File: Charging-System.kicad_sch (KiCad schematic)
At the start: 6 parts

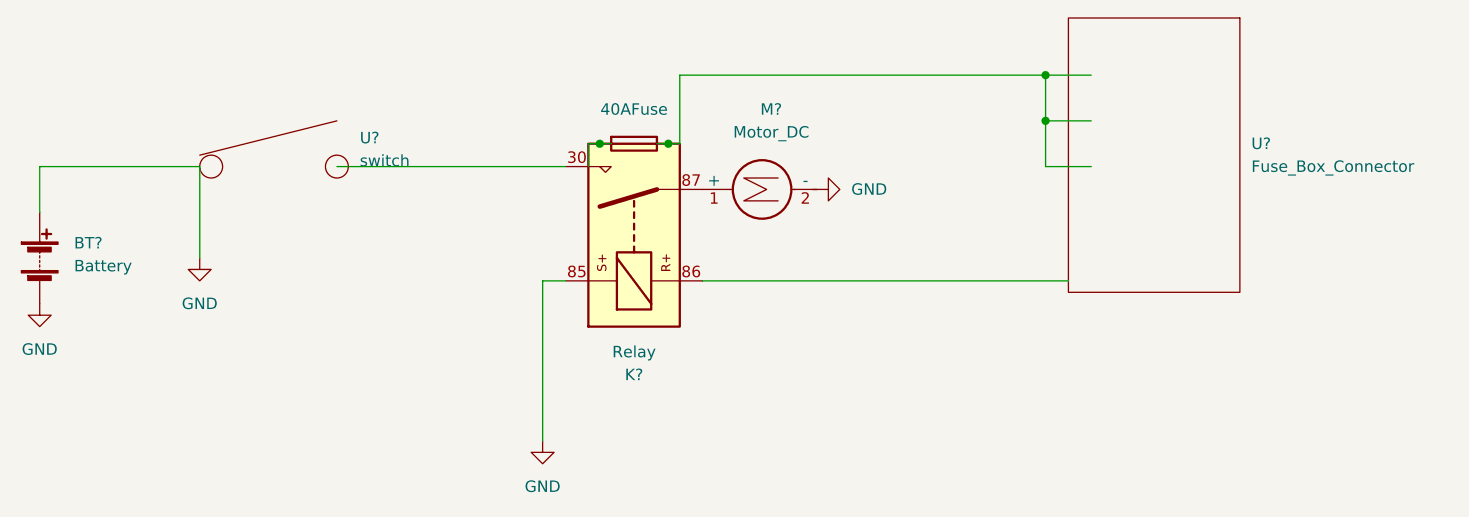
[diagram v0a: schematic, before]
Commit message: Changes to DTM Dash
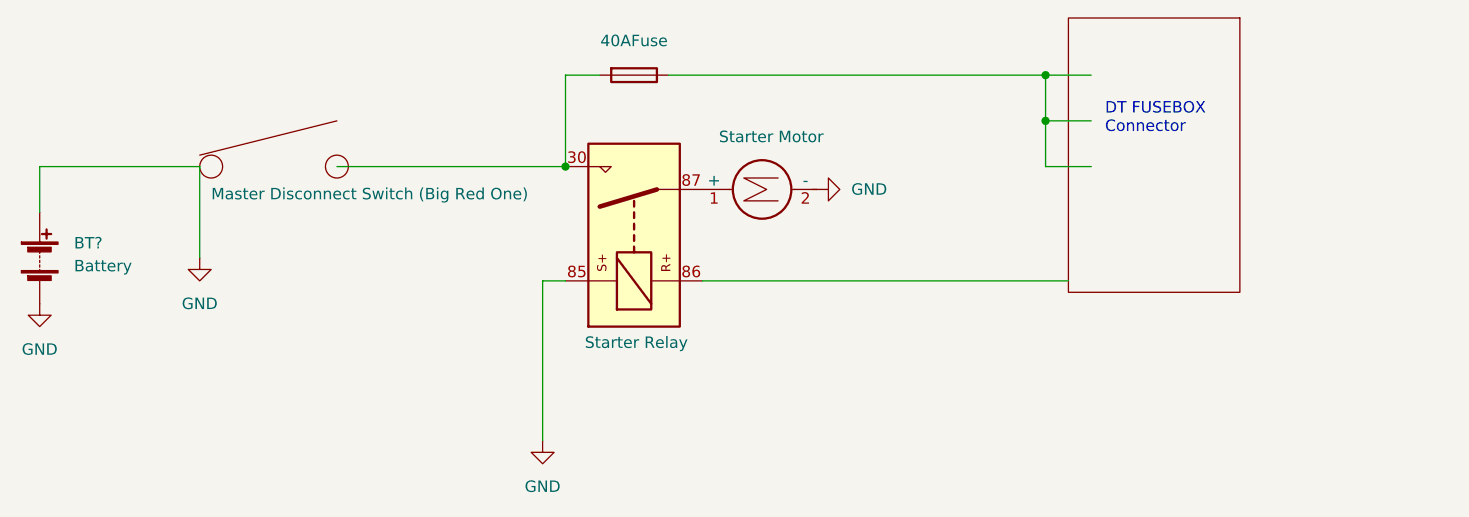
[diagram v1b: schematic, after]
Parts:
- K?: value Relay -> Starter Relay
- M?: value Motor_DC -> Starter Motor
- U?: value switch -> Master Disconnect Switch (Big Red One)
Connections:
- net at K?.30: now also F?.2
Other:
- note added: "DT FUSEBOX Connector"
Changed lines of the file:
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@@
   (junction (at 192.532 62.992) (diameter 0) (color 0 0 0 0)
   )
+  (junction (at 139.192 73.152) (diameter 0) (color 0 0 0 0)
+  )
   (junction (at 192.532 68.072) (diameter 0) (color 0 0 0 0)
-  )
-  (junction (at 150.622 70.612) (diameter 0) (color 0 0 0 0)
-  )
-  (junction (at 143.002 70.612) (diameter 0) (color 0 0 0 0)
   )
   (wire (pts (xy 197.612 73.152) (xy 192.532 73.152))
@@
     (stroke (width 0) (type default) (color 0 0 0 0))
   )
-  (wire (pts (xy 141.732 70.612) (xy 141.732 73.152))
-    (stroke (width 0) (type default) (color 0 0 0 0))
-  )
-  (wire (pts (xy 143.002 70.612) (xy 141.732 70.612))
-    (stroke (width 0) (type default) (color 0 0 0 0))
-  )
   (wire (pts (xy 136.652 85.852) (xy 136.652 103.632))
-    (stroke (width 0) (type default) (color 0 0 0 0))
-  )
-  (wire (pts (xy 150.622 70.612) (xy 151.892 70.612))
-    (stroke (width 0) (type default) (color 0 0 0 0))
-  )
-  (wire (pts (xy 149.352 70.612) (xy 150.622 70.612))
     (stroke (width 0) (type default) (color 0 0 0 0))
   )
@@
     (stroke (width 0) (type default) (color 0 0 0 0))
   )
-  (wire (pts (xy 113.792 73.152) (xy 139.192 73.152))
+  (wire (pts (xy 139.192 62.992) (xy 143.002 62.992))
     (stroke (width 0) (type default) (color 0 0 0 0))
   )
-  (wire (pts (xy 151.892 62.992) (xy 151.892 70.612))
+  (wire (pts (xy 113.792 73.152) (xy 139.192 73.152))
     (stroke (width 0) (type default) (color 0 0 0 0))
   )
@@
     (stroke (width 0) (type default) (color 0 0 0 0))
   )
-  (wire (pts (xy 144.272 70.612) (xy 143.002 70.612))
-    (stroke (width 0) (type default) (color 0 0 0 0))
-  )
-  (wire (pts (xy 151.892 62.992) (xy 192.532 62.992))
+  (wire (pts (xy 139.192 62.992) (xy 139.192 73.152))
     (stroke (width 0) (type default) (color 0 0 0 0))
   )
@@
     (stroke (width 0) (type default) (color 0 0 0 0))
   )
+  (wire (pts (xy 150.622 62.992) (xy 192.532 62.992))
+    (stroke (width 0) (type default) (color 0 0 0 0))
+  )
   (wire (pts (xy 139.192 85.852) (xy 136.652 85.852))
     (stroke (width 0) (type default) (color 0 0 0 0))
+  )
+  (text "DT FUSEBOX\nConnector\n" (at 199.136 69.596 0)
+    (effects (font (size 1.27 1.27)) (justify left bottom))
   )
   (symbol (lib_id "symbols:Fuse_Box_Connector") (at 205.232 70.612 270) (unit 1)
     (in_bom yes) (on_board yes) (fields_autoplaced)
     (property "Reference" "U?" (id 0) (at 215.392 70.6119 90)
-      (effects (font (size 1.27 1.27)) (justify left))
+      (effects (font (size 1.27 1.27)) (justify left) hide)
     )
-    (property "Value" "Fuse_Box_Connector" (id 1) (at 215.392 73.1519 90)
-      (effects (font (size 1.27 1.27)) (justify left))
+    (property "Value" "Fuse_Box_Connector" (id 1) (at 215.9 71.8819 90)
+      (effects (font (size 1.27 1.27)) (justify left) hide)
     )
     (property "Footprint" "" (id 2) (at 205.232 70.612 0)
@@
   )
   (symbol (lib_id "symbols:switch") (at 106.172 73.152 0) (unit 1)
-    (in_bom yes) (on_board yes) (fields_autoplaced)
-    (property "Reference" "U?" (id 0) (at 116.332 69.9769 0)
-      (effects (font (size 1.27 1.27)) (justify left))
+    (in_bom yes) (on_board yes)
+    (property "Reference" "U?" (id 0) (at 116.84 69.9769 0)
+      (effects (font (size 1.27 1.27)) (justify left) hide)
     )
-    (property "Value" "switch" (id 1) (at 116.332 72.5169 0)
+    (property "Value" "Master Disconnect Switch (Big Red One)" (id 1) (at 99.822 76.2 0)
       (effects (font (size 1.27 1.27)) (justify left))
     )
@@
   (symbol (lib_id "Motor:Motor_DC") (at 159.512 75.692 90) (unit 1)
     (in_bom yes) (on_board yes) (fields_autoplaced)
-    (property "Reference" "M?" (id 0) (at 162.052 66.802 90))
-    (property "Value" "Motor_DC" (id 1) (at 162.052 69.342 90))
+    (property "Reference" "M?" (id 0) (at 162.052 67.31 90)
+      (effects (font (size 1.27 1.27)) hide)
+    )
+    (property "Value" "Starter Motor" (id 1) (at 162.052 69.85 90))
     (property "Footprint" "" (id 2) (at 161.798 75.692 0)
       (effects (font (size 1.27 1.27)) hide)
@@
   )
   (symbol (lib_id "SCR23 Library:Relay") (at 146.7485 80.9117 180) (unit 1)
-    (in_bom yes) (on_board yes) (fields_autoplaced)
-    (property "Reference" "K?" (id 0) (at 146.812 96.2914 0))
-    (property "Value" "Relay" (id 1) (at 146.812 93.7514 0))
+    (in_bom yes) (on_board yes)
+    (property "Reference" "K?" (id 0) (at 146.812 64.77 0)
+      (effects (font (size 1.27 1.27)) hide)
+    )
+    (property "Value" "Starter Relay" (id 1) (at 147.066 92.71 0))
     (property "Footprint" "" (id 2) (at 113.0935 79.6417 0)
       (effects (font (size 1.27 1.27)) hide)
@@
     (pin "1")
   )
-  (symbol (lib_id "Device:Fuse") (at 146.812 70.612 270) (unit 1)
+  (symbol (lib_id "Device:Fuse") (at 146.812 62.992 270) (unit 1)
     (in_bom yes) (on_board yes) (fields_autoplaced)
-    (property "Reference" "F?" (id 0) (at 146.812 64.262 90)
+    (property "Reference" "F?" (id 0) (at 146.812 56.642 90)
       (effects (font (size 1.27 1.27)) hide)
     )
-    (property "Value" "40AFuse" (id 1) (at 146.812 66.802 90))
-    (property "Footprint" "" (id 2) (at 146.812 68.834 90)
+    (property "Value" "40AFuse" (id 1) (at 146.812 59.182 90))
+    (property "Footprint" "" (id 2) (at 146.812 61.214 90)
       (effects (font (size 1.27 1.27)) hide)
     )
-    (property "Datasheet" "~" (id 3) (at 146.812 70.612 0)
+    (property "Datasheet" "~" (id 3) (at 146.812 62.992 0)
       (effects (font (size 1.27 1.27)) hide)
     )

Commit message: Create new top level
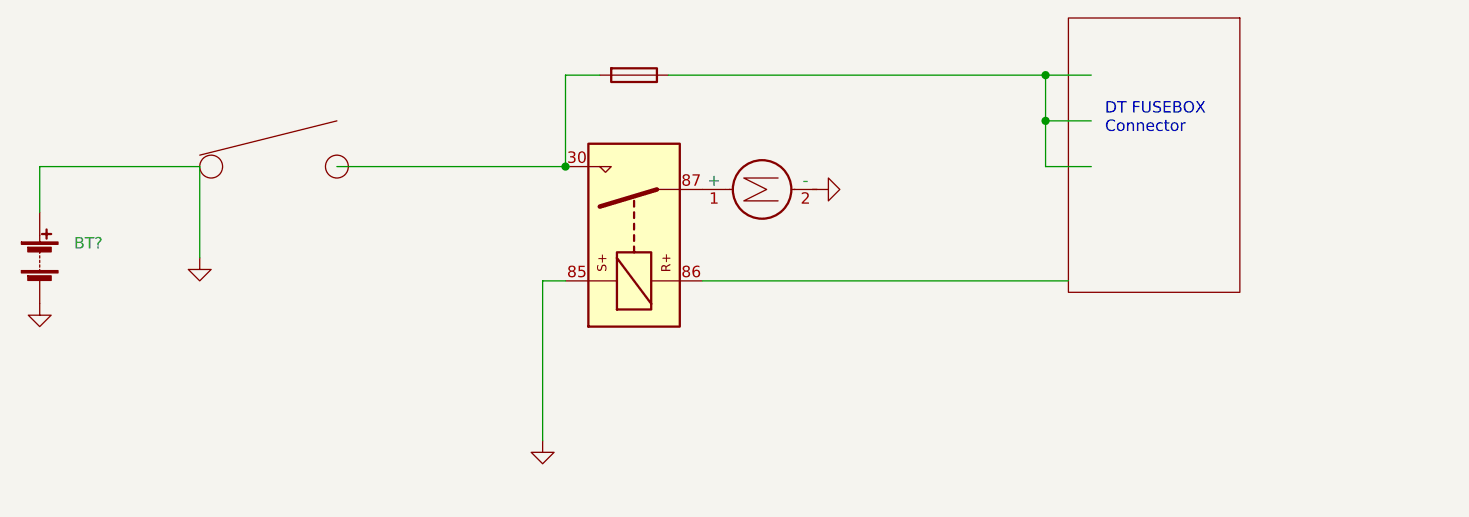
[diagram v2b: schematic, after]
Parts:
- BT?: value Battery -> (none)
- F?: value 40AFuse -> (none)
- K?: value Starter Relay -> (none)
- M?: value Starter Motor -> (none)
- U?: value Fuse_Box_Connector -> (none)
- U?: value Master Disconnect Switch (Big Red One) -> (none)
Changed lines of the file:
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@@
       (effects (font (size 1.27 1.27)) (justify left) hide)
     )
-    (property "Value" "Fuse_Box_Connector" (id 1) (at 215.9 71.8819 90)
+    (property "Value" "" (id 1) (at 215.9 71.8819 90)
       (effects (font (size 1.27 1.27)) (justify left) hide)
     )
@@
       (effects (font (size 1.27 1.27)) (justify left) hide)
     )
-    (property "Value" "Master Disconnect Switch (Big Red One)" (id 1) (at 99.822 76.2 0)
+    (property "Value" "" (id 1) (at 99.822 76.2 0)
       (effects (font (size 1.27 1.27)) (justify left))
     )
@@
       (effects (font (size 1.27 1.27)) hide)
     )
-    (property "Value" "GND" (id 1) (at 170.942 75.6919 90)
+    (property "Value" "" (id 1) (at 170.942 75.6919 90)
       (effects (font (size 1.27 1.27)) (justify right))
     )
@@
       (effects (font (size 1.27 1.27)) hide)
     )
-    (property "Value" "GND" (id 1) (at 80.772 93.472 0))
+    (property "Value" "" (id 1) (at 80.772 93.472 0))
     (property "Footprint" "" (id 2) (at 80.772 88.392 0)
       (effects (font (size 1.27 1.27)) hide)
@@
       (effects (font (size 1.27 1.27)) hide)
     )
-    (property "Value" "GND" (id 1) (at 98.552 88.392 0))
+    (property "Value" "" (id 1) (at 98.552 88.392 0))
     (property "Footprint" "" (id 2) (at 98.552 83.312 0)
       (effects (font (size 1.27 1.27)) hide)
@@
       (effects (font (size 1.27 1.27)) hide)
     )
-    (property "Value" "Starter Motor" (id 1) (at 162.052 69.85 90))
+    (property "Value" "" (id 1) (at 162.052 69.85 90))
     (property "Footprint" "" (id 2) (at 161.798 75.692 0)
       (effects (font (size 1.27 1.27)) hide)
@@
       (effects (font (size 1.27 1.27)) hide)
     )
-    (property "Value" "Starter Relay" (id 1) (at 147.066 92.71 0))
+    (property "Value" "" (id 1) (at 147.066 92.71 0))
     (property "Footprint" "" (id 2) (at 113.0935 79.6417 0)
       (effects (font (size 1.27 1.27)) hide)
@@
       (effects (font (size 1.27 1.27)) hide)
     )
-    (property "Value" "GND" (id 1) (at 136.652 108.712 0))
+    (property "Value" "" (id 1) (at 136.652 108.712 0))
     (property "Footprint" "" (id 2) (at 136.652 103.632 0)
       (effects (font (size 1.27 1.27)) hide)
@@
       (effects (font (size 1.27 1.27)) hide)
     )
-    (property "Value" "40AFuse" (id 1) (at 146.812 59.182 90))
+    (property "Value" "" (id 1) (at 146.812 59.182 90))
     (property "Footprint" "" (id 2) (at 146.812 61.214 90)
       (effects (font (size 1.27 1.27)) hide)
@@
       (effects (font (size 1.27 1.27)) (justify left))
     )
-    (property "Value" "Battery" (id 1) (at 84.582 84.2009 0)
+    (property "Value" "" (id 1) (at 84.582 84.2009 0)
       (effects (font (size 1.27 1.27)) (justify left))
     )

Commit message: HUGE TOP LEVEL
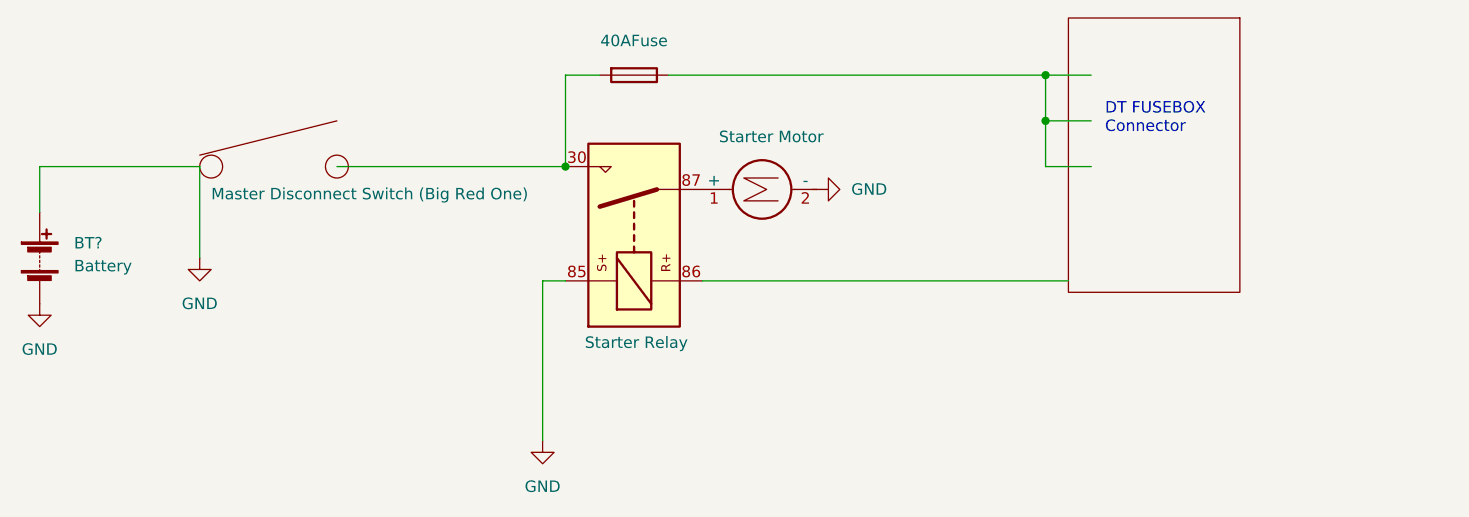
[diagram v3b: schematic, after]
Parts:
- BT?: value (none) -> Battery
- F?: value (none) -> 40AFuse
- K?: value (none) -> Starter Relay
- M?: value (none) -> Starter Motor
- U?: value (none) -> Fuse_Box_Connector
- U?: value (none) -> Master Disconnect Switch (Big Red One)
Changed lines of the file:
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@@
       (effects (font (size 1.27 1.27)) (justify left) hide)
     )
-    (property "Value" "" (id 1) (at 215.9 71.8819 90)
+    (property "Value" "Fuse_Box_Connector" (id 1) (at 215.9 71.8819 90)
       (effects (font (size 1.27 1.27)) (justify left) hide)
     )
@@
       (effects (font (size 1.27 1.27)) (justify left) hide)
     )
-    (property "Value" "" (id 1) (at 99.822 76.2 0)
+    (property "Value" "Master Disconnect Switch (Big Red One)" (id 1) (at 99.822 76.2 0)
       (effects (font (size 1.27 1.27)) (justify left))
     )
@@
       (effects (font (size 1.27 1.27)) hide)
     )
-    (property "Value" "" (id 1) (at 170.942 75.6919 90)
+    (property "Value" "GND" (id 1) (at 170.942 75.6919 90)
       (effects (font (size 1.27 1.27)) (justify right))
     )
@@
       (effects (font (size 1.27 1.27)) hide)
     )
-    (property "Value" "" (id 1) (at 80.772 93.472 0))
+    (property "Value" "GND" (id 1) (at 80.772 93.472 0))
     (property "Footprint" "" (id 2) (at 80.772 88.392 0)
       (effects (font (size 1.27 1.27)) hide)
@@
       (effects (font (size 1.27 1.27)) hide)
     )
-    (property "Value" "" (id 1) (at 98.552 88.392 0))
+    (property "Value" "GND" (id 1) (at 98.552 88.392 0))
     (property "Footprint" "" (id 2) (at 98.552 83.312 0)
       (effects (font (size 1.27 1.27)) hide)
@@
       (effects (font (size 1.27 1.27)) hide)
     )
-    (property "Value" "" (id 1) (at 162.052 69.85 90))
+    (property "Value" "Starter Motor" (id 1) (at 162.052 69.85 90))
     (property "Footprint" "" (id 2) (at 161.798 75.692 0)
       (effects (font (size 1.27 1.27)) hide)
@@
       (effects (font (size 1.27 1.27)) hide)
     )
-    (property "Value" "" (id 1) (at 147.066 92.71 0))
+    (property "Value" "Starter Relay" (id 1) (at 147.066 92.71 0))
     (property "Footprint" "" (id 2) (at 113.0935 79.6417 0)
       (effects (font (size 1.27 1.27)) hide)
@@
       (effects (font (size 1.27 1.27)) hide)
     )
-    (property "Value" "" (id 1) (at 136.652 108.712 0))
+    (property "Value" "GND" (id 1) (at 136.652 108.712 0))
     (property "Footprint" "" (id 2) (at 136.652 103.632 0)
       (effects (font (size 1.27 1.27)) hide)
@@
       (effects (font (size 1.27 1.27)) hide)
     )
-    (property "Value" "" (id 1) (at 146.812 59.182 90))
+    (property "Value" "40AFuse" (id 1) (at 146.812 59.182 90))
     (property "Footprint" "" (id 2) (at 146.812 61.214 90)
       (effects (font (size 1.27 1.27)) hide)
@@
       (effects (font (size 1.27 1.27)) (justify left))
     )
-    (property "Value" "" (id 1) (at 84.582 84.2009 0)
+    (property "Value" "Battery" (id 1) (at 84.582 84.2009 0)
       (effects (font (size 1.27 1.27)) (justify left))
     )
